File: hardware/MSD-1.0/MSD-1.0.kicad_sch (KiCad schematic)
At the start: 25 parts, among them J1 Conn_01x05, J2 Conn_01x03, Q1 IRF840, U1 NE555P, U2 PC817, U3 PC817

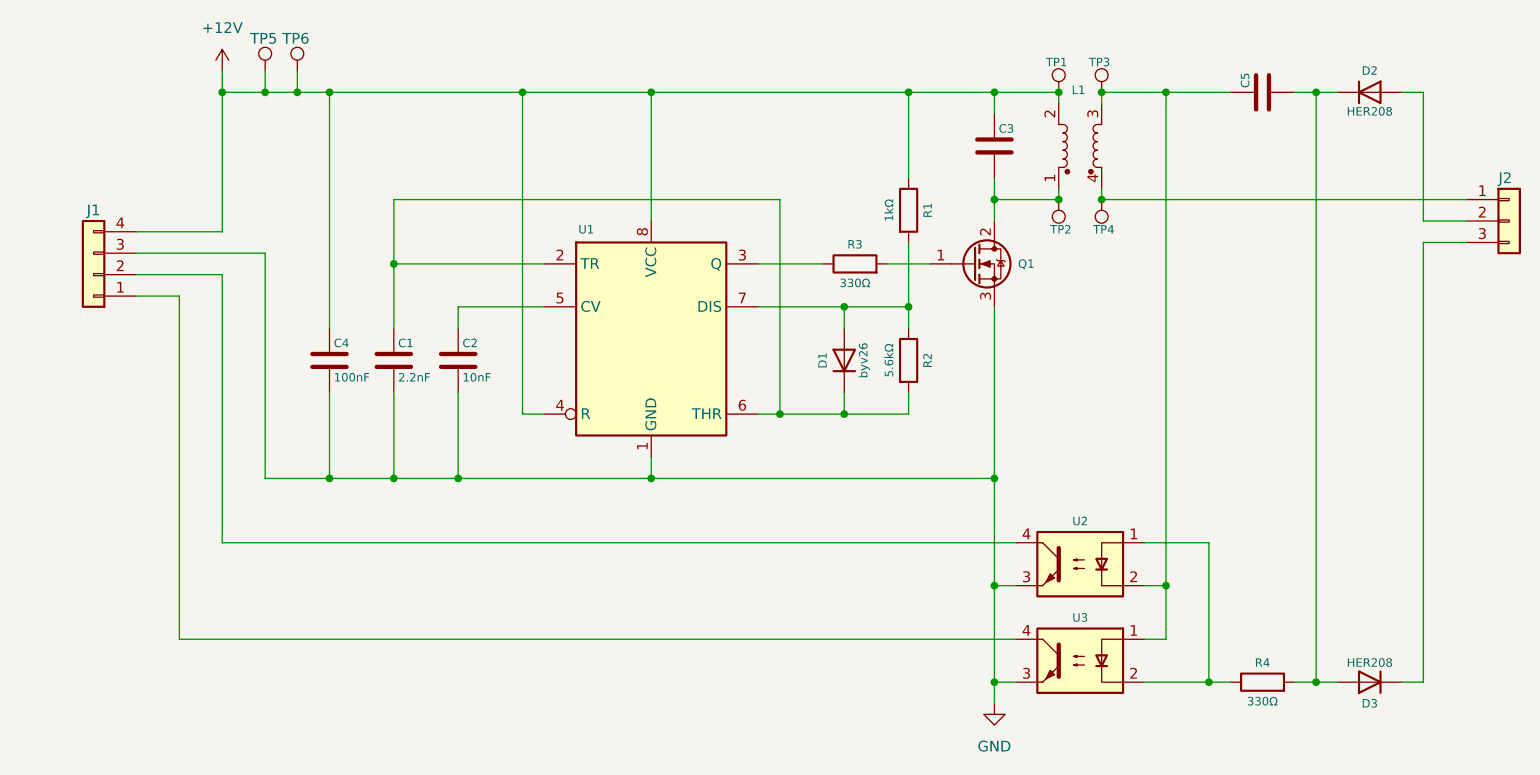
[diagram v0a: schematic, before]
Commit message: modified:   .DS_Store 	deleted:    hardware/MSD-1.0/MSD-1.0-backups/MSD-1.0-2025-02-25_161819.zip 	deleted:    hardware/MSD-1.0/MSD-1.0-backups/MSD-1.0-2025-02-25_162448.zip 	deleted:    hardware/MSD-1.0/MSD-1.0-backups/MSD-1.0-2025-02-25_163016.zip 	deleted:    hardware/MSD-1.0/MSD-1.0-backups/MSD-1.0-2025-02-25_163954.zip 	deleted:    hardware/MSD-1.0/MSD-1.0-backups/MSD-1.0-2025-02-26_112856.zip 	deleted:    hardware/MSD-1.0/MSD-1.0-backups/MSD-1.0-2025-02-26_113923.zip 	deleted:    hardware/MSD-1.0/MSD-1.0-backups/MSD-1.0-2025-02-26_115654.zip 	deleted:    hardware/MSD-1.0/MSD-1.0-backups/MSD-1.0-2025-02-26_120757.zip 	deleted:    hardware/MSD-1.0/MSD-1.0-backups/MSD-1.0-2025-02-26_163854.zip 	deleted:    hardware/MSD-1.0/MSD-1.0-backups/MSD-1.0-2025-02-27_112851.zip 	deleted:    hardware/MSD-1.0/MSD-1.0-backups/MSD-1.0-2025-02-27_114053.zip 	deleted:    hardware/MSD-1.0/MSD-1.0-backups/MSD-1.0-2025-02-27_185834.zip 	deleted:    hardware/MSD-1.0/MSD-1.0-backups/MSD-1.0-2025-02-27_190654.zip 	deleted:    hardware/MSD-1.0/MSD-1.0-backups/MSD-1.0-2025-02-27_191228.zip 	deleted:    hardware/MSD-1.0/MSD-1.0-backups/MSD-1.0-2025-02-28_140545.zip 	deleted:    hardware/MSD-1.0/MSD-1.0-backups/MSD-1.0-2025-02-28_141533.zip 	deleted:    hardware/MSD-1.0/MSD-1.0-backups/MSD-1.0-2025-02-28_142536.zip 	deleted:    hardware/MSD-1.0/MSD-1.0-backups/MSD-1.0-2025-02-28_143342.zip 	deleted:    hardware/MSD-1.0/MSD-1.0-backups/MSD-1.0-2025-02-28_162722.zip 	deleted:    hardware/MSD-1.0/MSD-1.0-backups/MSD-1.0-2025-03-05_134102.zip 	deleted:    hardware/MSD-1.0/MSD-1.0-backups/MSD-1.0-2025-03-05_134620.zip 	new file:   hardware/MSD-1.0/MSD-1.0-backups/MSD-1.0-2025-03-24_113503.zip 	new file:   hardware/MSD-1.0/MSD-1.0-backups/MSD-1.0-2025-03-24_114029.zip 	new file:   hardware/MSD-1.0/MSD-1.0-backups/MSD-1.0-2025-03-24_132745.zip 	new file:   hardware/MSD-1.0/MSD-1.0-backups/MSD-1.0-2025-03-24_134332.zip 	new file:   hardware/MSD-1.0/MSD-1.0-backups/MSD-1.0-2025-03-25_144744.zip 	n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
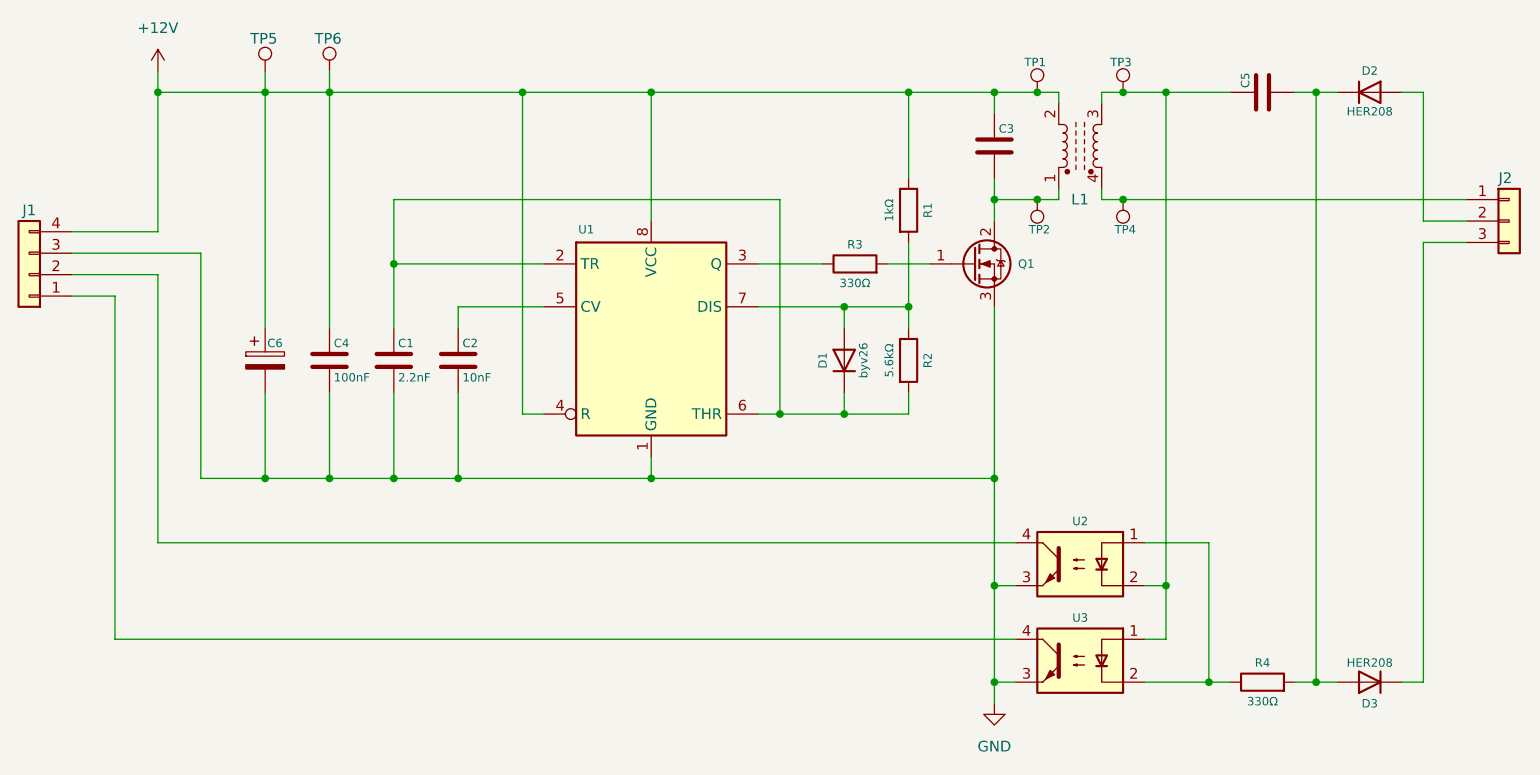
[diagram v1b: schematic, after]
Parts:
- removed L1: Isolation Transformer (Custom), Inductor_THT:L_CommonMode_Toroid_Vertical_L30.5mm_W15.2mm_Px10.16mm_Py20.32mm_Bourns_8100, symbol Device:L_Coupled_1243
- added C6: 470µF 35V, Capacitor_THT:CP_Radial_D12.5mm_P5.00mm, symbol Device:C_Polarized
- added L1: L_Ferrite_Coupled, Inductor_THT:L_CommonMode_Toroid_Horizontal_OD23mm_ID14mm_H8mm, symbol Device:L_Ferrite_Coupled_1243
- D1: footprint Diode_THT:D_DO-34_SOD68_P7.62mm_Horizontal -> Diode_THT:D_DO-35_SOD27_P7.62mm_Horizontal
- J1: footprint Connector_PinHeader_2.54mm:PinHeader_1x04_P2.54mm_Horizontal_Custom -> Connector_PinHeader_2.54mm:PinHeader_1x04_P2.54mm_Horizontal_2
- J2: footprint Connector_PinHeader_2.54mm:PinHeader_1x03_P5.08mm_Horizontal_Custom -> Connector_PinHeader_2.54mm:PinHeader_1x03_P5.08mm_Horizontal_2
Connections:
- net +12V: now also C6.1, L1.2
- net GND: now also C6.2
- net at C3.2, Q1.2 (D), TP2.1: now also L1.1
- net at J2.1 (Pin_1), TP4.1: now also L1.4
- net at C5.1, TP3.1, U2.2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: now also L1.3
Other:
- moved on the sheet: J1, TP1, TP2, TP3, TP4, TP6
